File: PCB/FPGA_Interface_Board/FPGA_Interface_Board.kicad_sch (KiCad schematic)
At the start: 23 parts, among them J1 USB_B_Micro, J2 Conn_01x02_Pin, J3 Conn_01x04_Socket, U1 MCP2200-I-SS, U2 MCP4822, U3 PAM8302AAS, Y1 12MHz

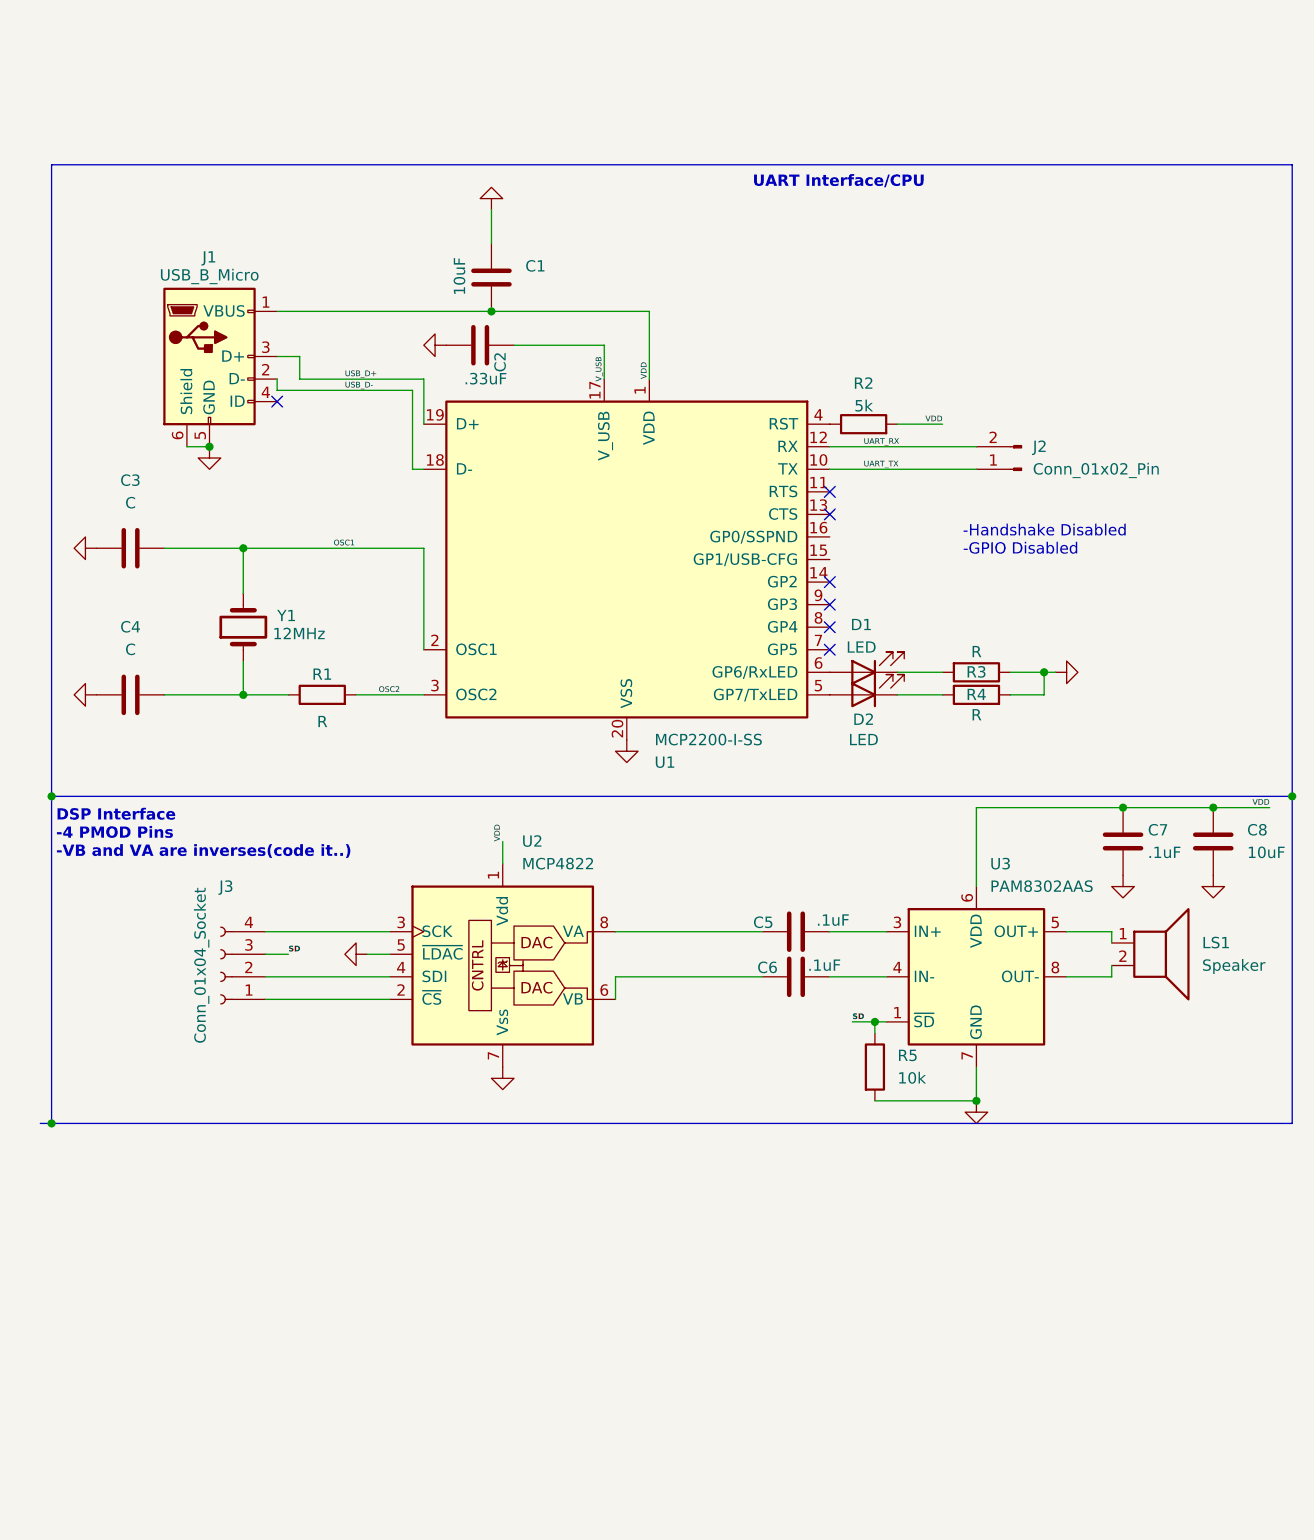
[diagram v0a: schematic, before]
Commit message: got sim to work on fft
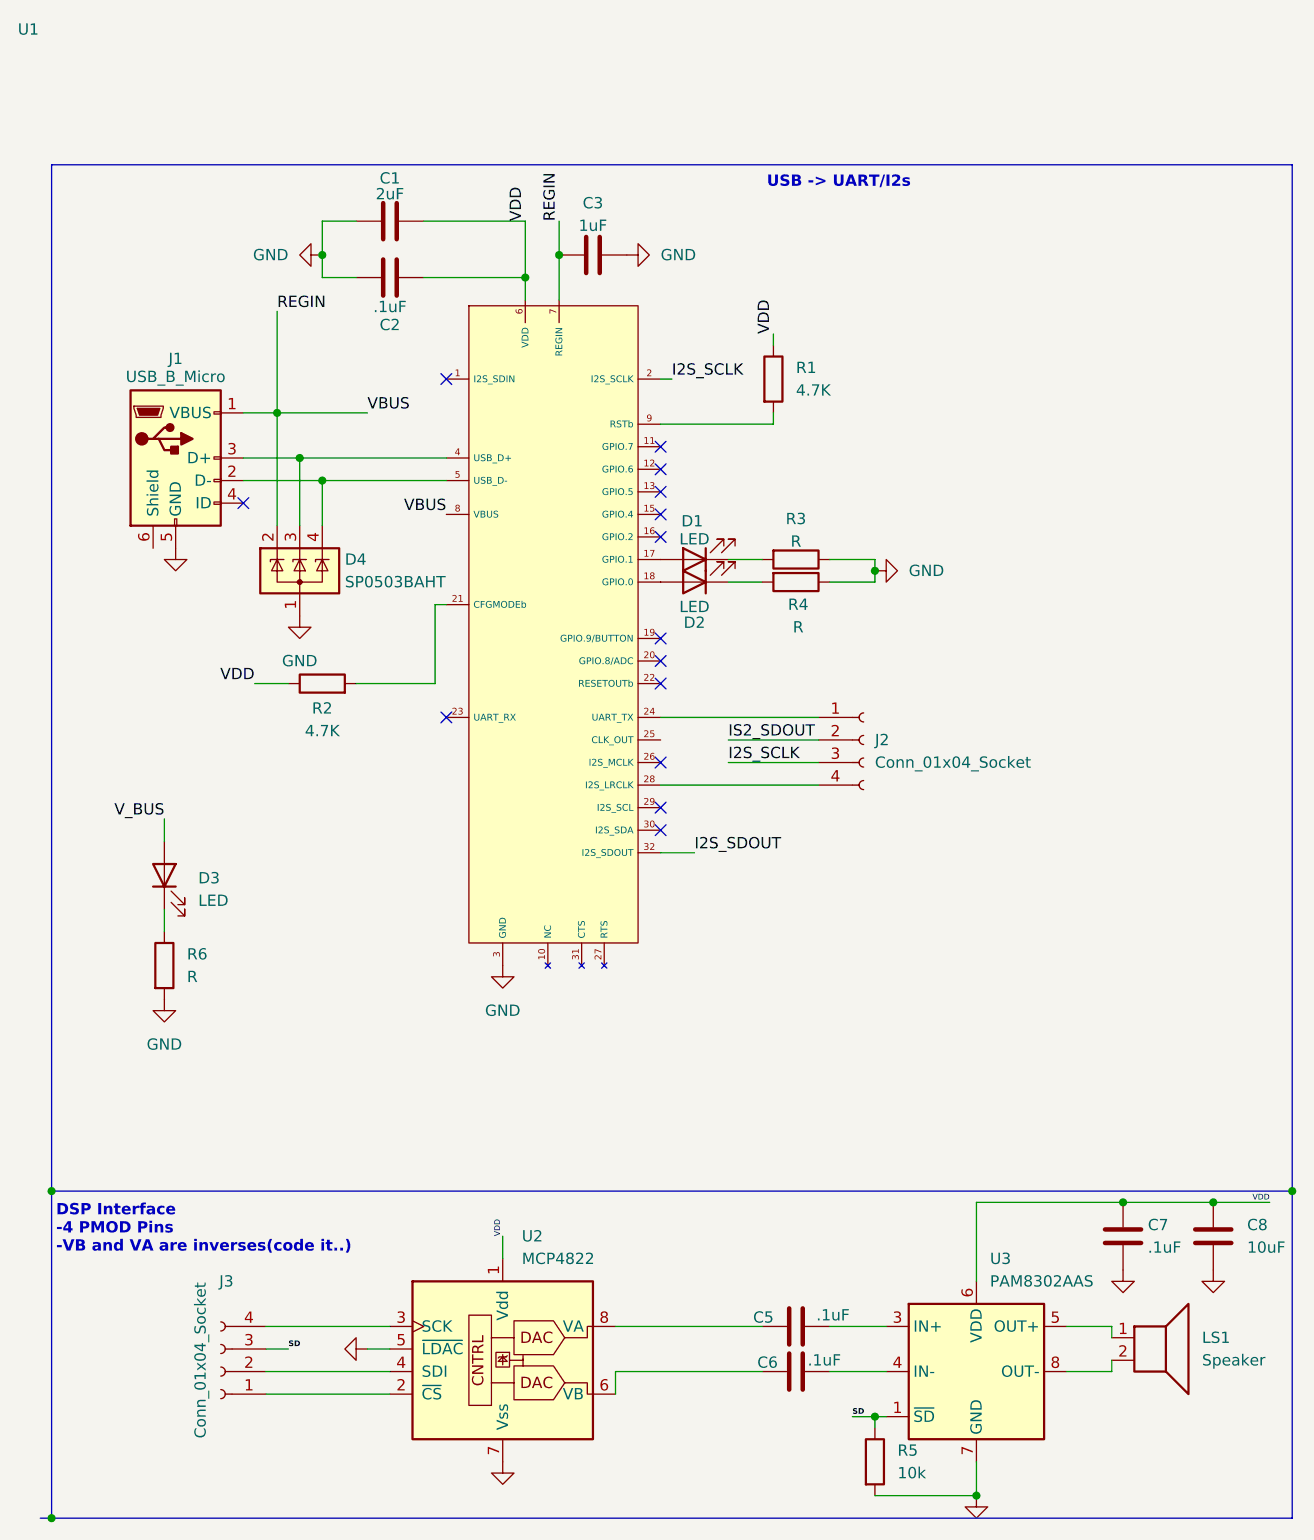
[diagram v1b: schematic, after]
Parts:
- removed C4: C, symbol Device:C
- removed J2: Conn_01x02_Pin, Connector_Samtec_HPM_THT:Samtec_HPM-02-01-x-S_Straight_1x02_Pitch5.08mm, symbol Connector:Conn_01x02_Pin
- removed U1: MCP2200-I-SS, Package_SO:SSOP-20_5.3x7.2mm_P0.65mm, symbol Interface_USB:MCP2200-I-SS
- removed Y1: 12MHz, symbol Device:Crystal
- added D3: LED, symbol Device:LED
- added D4: SP0503BAHT, Package_TO_SOT_SMD:SOT-143, symbol Power_Protection:SP0503BAHT
- added J2: Conn_01x04_Socket, symbol Connector:Conn_01x04_Socket
- added R6: R, symbol Device:R
- added U1, U4: ~, symbol SOC:U-CP2615-A02
- C1: value 10uF -> 2uF
- C2: value .33uF -> .1uF
- C3: value C -> 1uF
- R1: value R -> 4.7K
- R2: value 5k -> 4.7K
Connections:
- net OSC1 is gone; now on net GND: C3.2
- net V_USB is gone; now on net GND: C2.2
- net GND: now also R4.1, D4.1 (A), R6.2, U4.3 (GND); no longer C2.1, C3.1, J1.6 (Shield), R4.2
- net VDD: now also C2.1, R1.1, R2.1, U4.6 (VDD); no longer J1.1 (VBUS), R2.2
- net at D2.2 (A): now also U4.18 (GPIO.0)
- net at D1.2 (A): now also U4.17 (GPIO.1)
- net at D2.1 (K): now also R4.2; no longer R4.1
- net OSC2: no longer names the net of R1.2
- net OSC2: now also U4.9 (RSTb)
- net USB_D+: no longer names the net of J1.3 (D+)
- net USB_D+: now also D4.3 (K), U4.4 (USB_D+)
- net USB_D-: no longer names the net of J1.2 (D-)
- net USB_D-: now also D4.4 (K), U4.5 (USB_D-)
- new net: R2.2, U4.21 (CFGMODEb)
- new net: J2.1 (Pin_1), U4.24 (UART_TX)
- new net: J2.4 (Pin_4), U4.28 (I2S_LRCLK)
- new net: D3.1 (K), R6.1
- new net I2S_SCLK: J2.3 (Pin_3), U4.2 (I2S_SCLK)
- new net I2S_SDOUT: U4.32 (I2S_SDOUT)
- new net IS2_SDOUT: J2.2 (Pin_2)
- new net REGIN: C3.1, D4.2 (K), J1.1 (VBUS), U4.7 (REGIN), U4.8 (VBUS)
- new net V_BUS: D3.2 (A)
- no-connect marks 7 -> 14
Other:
- note added: "USB -> UART/I2s"
- note removed: "-Handshake Disabled -GPIO Disabled"
- note removed: "UART Interface/CPU"
- moved on the sheet: C5, C6, C7, C8, J1, J3, LS1, R5, U2, U3
